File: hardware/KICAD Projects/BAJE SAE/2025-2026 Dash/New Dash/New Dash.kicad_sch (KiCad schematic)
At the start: 5 parts, among them J1 CAN to outer connector, J999 Conn_01x06, U1 XIAO-ESP32-S3-SMD

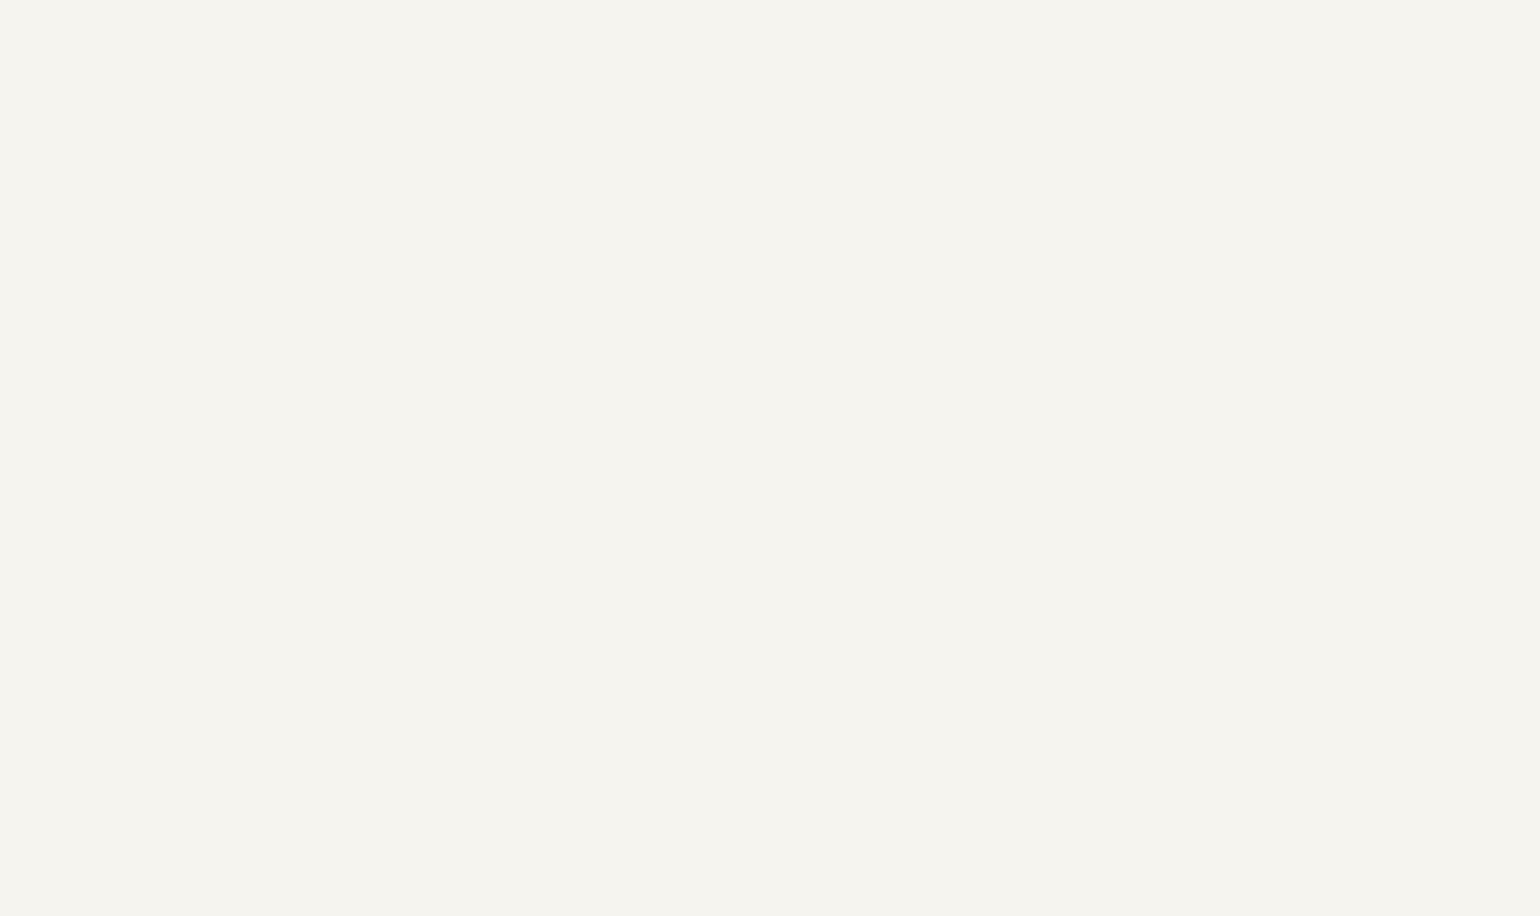
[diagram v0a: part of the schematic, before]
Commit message: Pasted in Connectors
Added Servo Connectors
Button connectors
socket
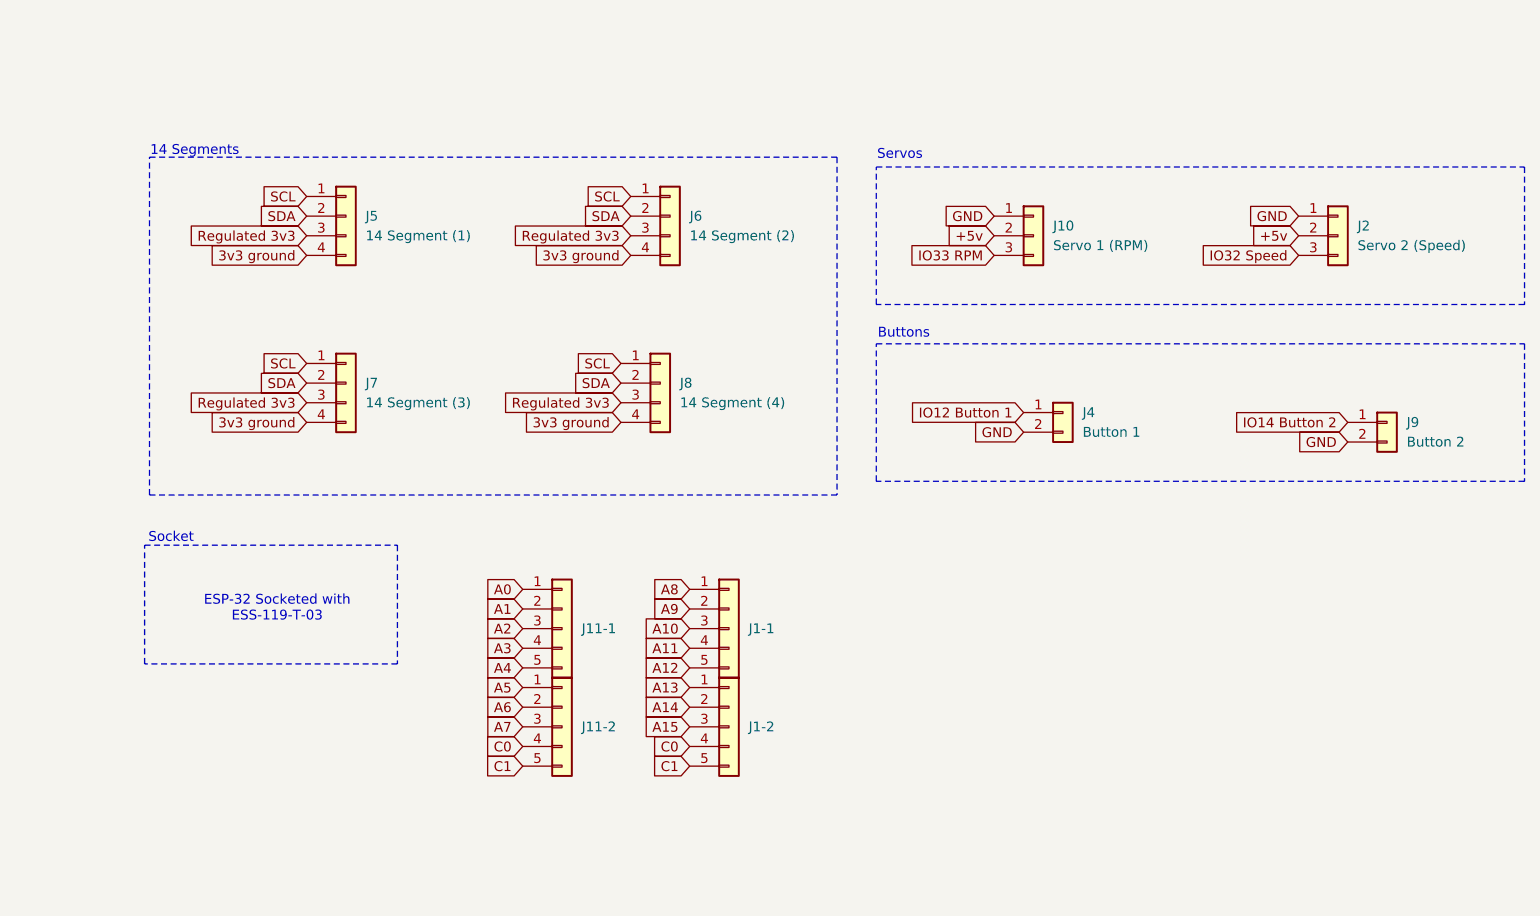
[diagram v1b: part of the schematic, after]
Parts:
- added J1-1, J1-2, J11-1, J11-2: Conn_01x05, Connector_PinHeader_2.54mm:PinHeader_1x05_P2.54mm_Vertical, symbol Connector_Generic:Conn_01x05
- added J10: Servo 1 (RPM), Connector_PinHeader_2.54mm:PinHeader_1x03_P2.54mm_Vertical, symbol Connector_Generic:Conn_01x03
- added J2: Servo 2 (Speed), Connector_PinHeader_2.54mm:PinHeader_1x03_P2.54mm_Vertical, symbol Connector_Generic:Conn_01x03
- added J4: Button 1, Connector_PinHeader_2.54mm:PinHeader_1x02_P2.54mm_Vertical, symbol Connector_Generic:Conn_01x02
- added J5: 14 Segment (1), Connector_PinHeader_2.54mm:PinHeader_1x04_P2.54mm_Vertical, symbol Connector_Generic:Conn_01x04
- added J6: 14 Segment (2), Connector_PinHeader_2.54mm:PinHeader_1x04_P2.54mm_Vertical, symbol Connector_Generic:Conn_01x04
- added J7: 14 Segment (3), Connector_PinHeader_2.54mm:PinHeader_1x04_P2.54mm_Vertical, symbol Connector_Generic:Conn_01x04
- added J8: 14 Segment (4), Connector_PinHeader_2.54mm:PinHeader_1x04_P2.54mm_Vertical, symbol Connector_Generic:Conn_01x04
- added J9: Button 2, Connector_PinHeader_2.54mm:PinHeader_1x02_P2.54mm_Vertical, symbol Connector_Generic:Conn_01x02
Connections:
- net +5v: now also J10.2 (Pin_2), J2.2 (Pin_2)
- net 3v3 ground: now also J5.4 (Pin_4), J6.4 (Pin_4), J7.4 (Pin_4), J8.4 (Pin_4)
- net A0: now also J11-1.1 (Pin_1)
- net A1: now also J11-1.2 (Pin_2)
- net A10: now also J1-1.3 (Pin_3)
- net A11: now also J1-1.4 (Pin_4)
- net A12: now also J1-1.5 (Pin_5)
- net A13: now also J1-2.1 (Pin_1)
- net A14: now also J1-2.2 (Pin_2)
- net A15: now also J1-2.3 (Pin_3)
- net A2: now also J11-1.3 (Pin_3)
- net A3: now also J11-1.4 (Pin_4)
- net A4: now also J11-1.5 (Pin_5)
- net A5: now also J11-2.1 (Pin_1)
- net A6: now also J11-2.2 (Pin_2)
- net A7: now also J11-2.3 (Pin_3)
- net A8: now also J1-1.1 (Pin_1)
- net A9: now also J1-1.2 (Pin_2)
- net C0: now also J1-2.4 (Pin_4), J11-2.4 (Pin_4)
- net C1: now also J1-2.5 (Pin_5), J11-2.5 (Pin_5)
- net GND: now also J10.1 (Pin_1), J2.1 (Pin_1), J4.2 (Pin_2), J9.2 (Pin_2)
- net Regulated 3v3: now also J5.3 (Pin_3), J6.3 (Pin_3), J7.3 (Pin_3), J8.3 (Pin_3)
- net SCL: now also J5.1 (Pin_1), J6.1 (Pin_1), J7.1 (Pin_1), J8.1 (Pin_1)
- net SDA: now also J5.2 (Pin_2), J6.2 (Pin_2), J7.2 (Pin_2), J8.2 (Pin_2)
- new net IO12 Button 1: J4.1 (Pin_1)
- new net IO14 Button 2: J9.1 (Pin_1)
- new net IO32 Speed: J2.3 (Pin_3)
- new net IO33 RPM: J10.3 (Pin_3)
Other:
- note added: "14 Segments"
- note added: "Buttons"
- note added: "ESP-32 Socketed with ESS-119-T-03"
- note added: "Servos"
- note added: "Socket"
